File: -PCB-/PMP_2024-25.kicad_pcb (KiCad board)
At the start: 2 copper layers, 123 x 55.5 mm, 49 parts, among them J1 OUT, J2 5V, J3 GND, J4 CALIB, Q1 NPN 2N3904, Q2 NPN 2N3904, Q3 NPN MPSA42, Q4 NPN 2N3904

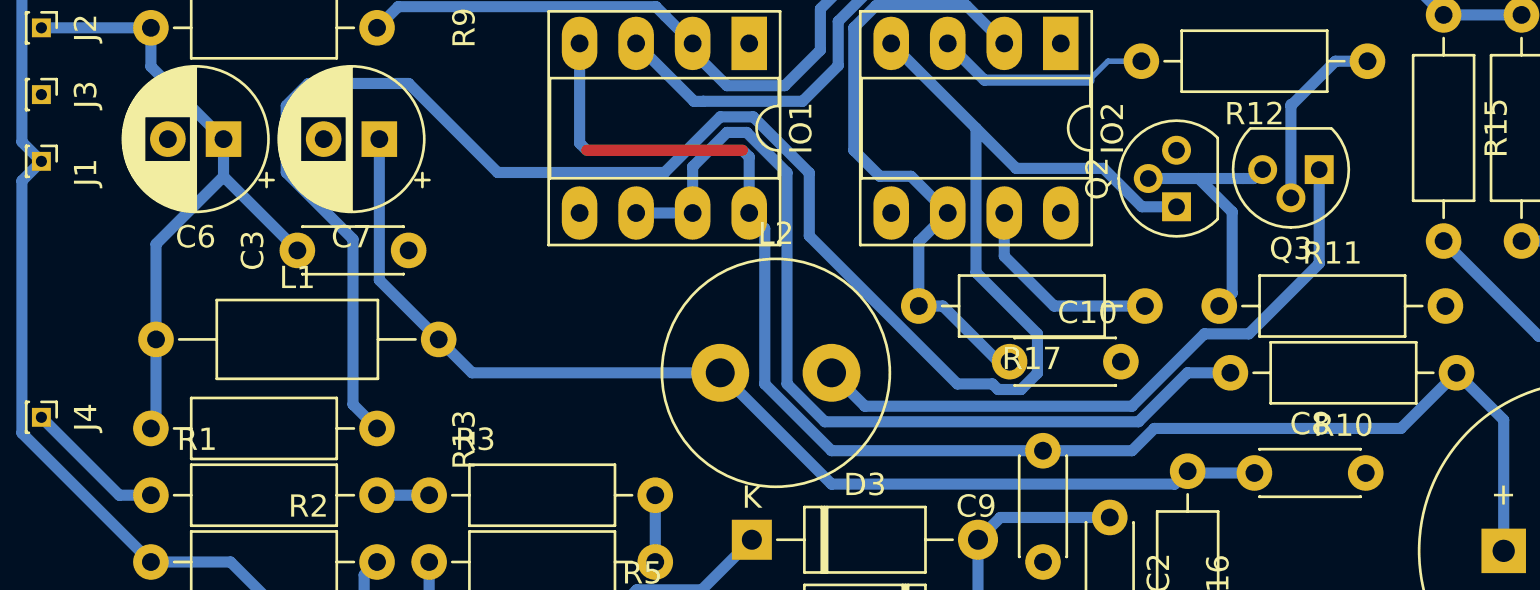
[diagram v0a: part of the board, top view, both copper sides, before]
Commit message: some edits
excel added too
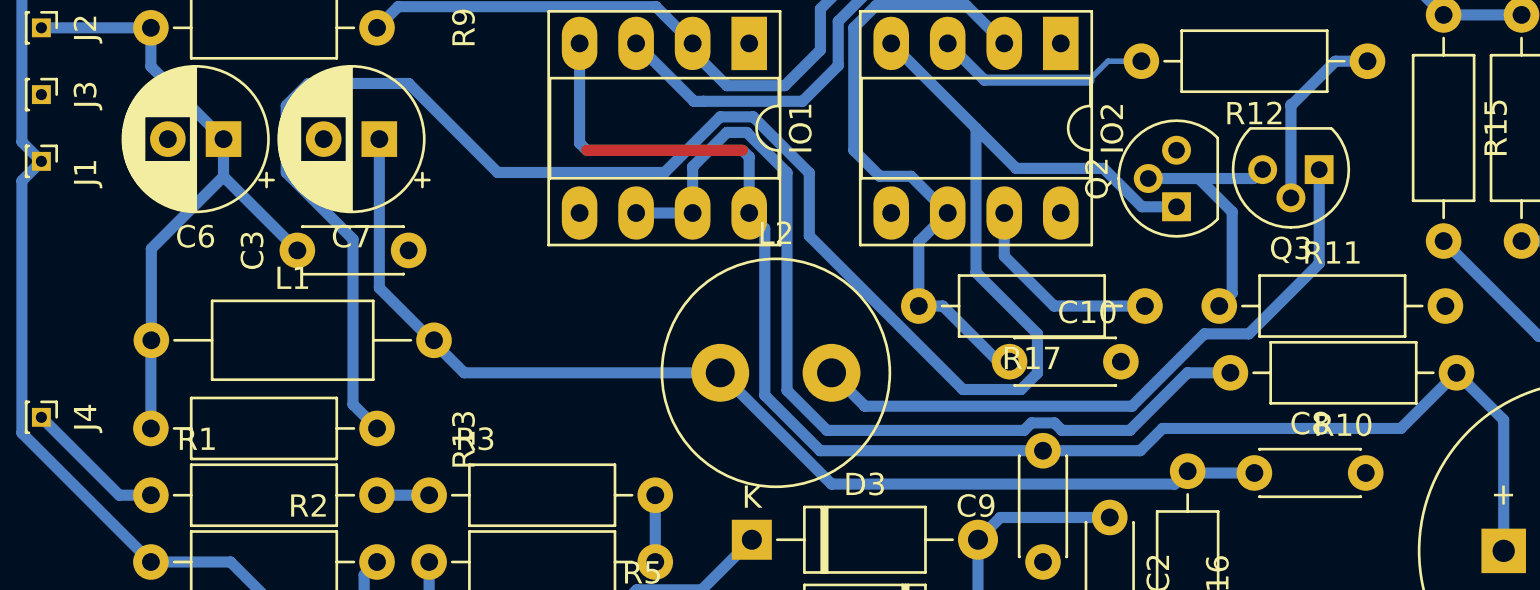
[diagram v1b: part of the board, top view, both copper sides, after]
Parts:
- moved L1 0.21 mm to (67.9, 65.0)
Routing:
- net Net-(IO1-DIS): track 41.3 -> 42.0 mm
- net VCC: track 30.3 -> 31.0 mm

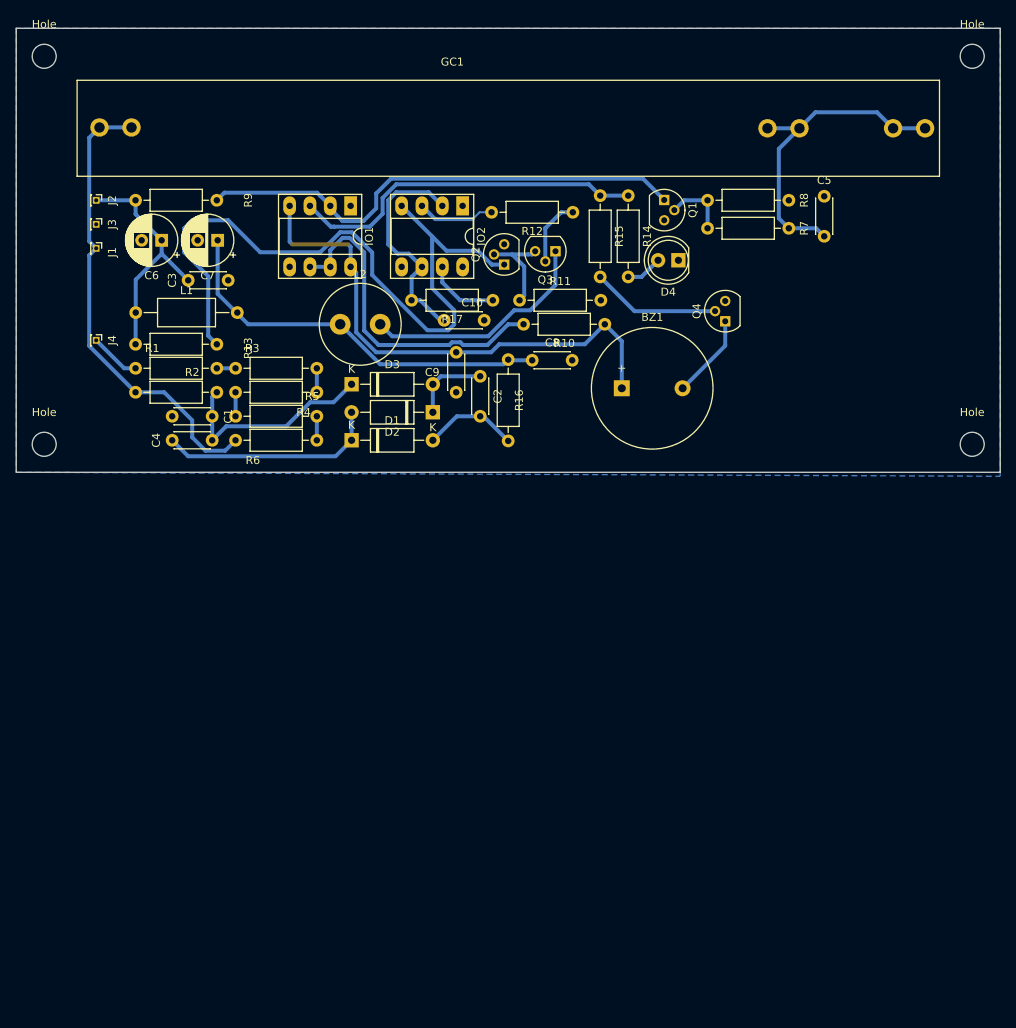
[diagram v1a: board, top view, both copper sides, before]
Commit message: PCB update
V2
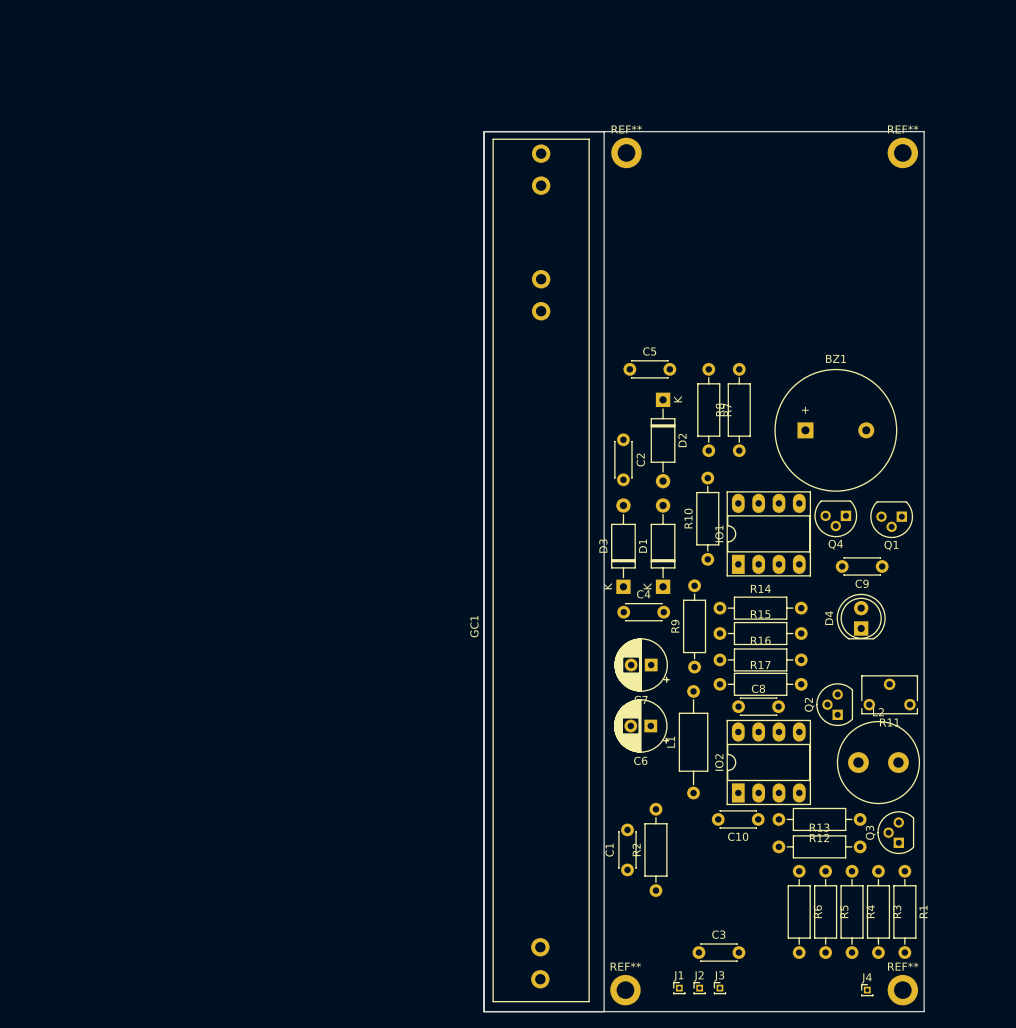
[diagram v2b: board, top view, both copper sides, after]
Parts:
- removed Hole (x4): MountingHole_3mm, MountingHole:MountingHole_3mm
- added REF**: MountingHole_2.2mm_M2_DIN965_Pad, MountingHole:MountingHole_2.2mm_M2_DIN965_Pad, F.Cu at (163.8, 149.7)
- added REF**: MountingHole_2.2mm_M2_DIN965_Pad, MountingHole:MountingHole_2.2mm_M2_DIN965_Pad, F.Cu at (129.2, 149.7)
- added REF**: MountingHole_2.2mm_M2_DIN965_Pad, MountingHole:MountingHole_2.2mm_M2_DIN965_Pad, F.Cu at (163.8, 45.1)
- added REF**: MountingHole_2.2mm_M2_DIN965_Pad, MountingHole:MountingHole_2.2mm_M2_DIN965_Pad, F.Cu at (129.3, 45.1)
- J4: value CALIB -> TEST
- R11: footprint Resistor_THT:R_Axial_DIN0207_L6.3mm_D2.5mm_P10.16mm_Horizontal -> Potentiometer_THT:Potentiometer_Bourns_3266W_Vertical
- R14: value ? -> 1k
- moved J4 126.1 mm to (159.4, 149.7), turned to 0 degrees
- moved J2 124.0 mm to (138.4, 149.5), turned to 0 degrees
- moved J3 123.3 mm to (141.0, 149.5), turned to 0 degrees
- moved GC1 123.2 mm to (119.6, 151.2), turned to 90 degrees
- moved J1 117.8 mm to (135.9, 149.5), turned to 0 degrees
- moved R1 106.5 mm to (164.1, 134.9), turned to -90 degrees
- moved C3 105.5 mm to (138.3, 145.0)
- moved R13 102.0 mm to (148.3, 131.8)
- moved R3 102.0 mm to (160.8, 134.9), turned to -90 degrees
- moved R4 97.6 mm to (157.5, 134.9), turned to -90 degrees
- moved R5 93.1 mm to (154.2, 134.9), turned to -90 degrees
- moved L1 92.0 mm to (137.7, 125.1), turned to 90 degrees
- moved R9 91.0 mm to (137.8, 109.3), turned to 90 degrees
- moved R2 90.1 mm to (133.0, 137.3), turned to 90 degrees
- moved R6 88.7 mm to (150.9, 134.9), turned to -90 degrees
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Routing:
- net RES: track 88.1 -> 0.00 mm
- net TRIG: track 62.4 -> 0.00 mm
- net Net-(BZ1-+): track 58.4 -> 0.00 mm
- net CALIB: track 58.1 -> 0.00 mm
- net Net-(IO2-VCC): track 50.1 -> 0.00 mm
- net Net-(IO1-Q): track 44.8 -> 0.00 mm
- net Net-(IO1-DIS): track 42.0 -> 0.00 mm
- net Net-(C5-Pad2): track 40.3 -> 0.00 mm
- net VCC: track 31.0 -> 0.06 mm
- net Net-(Q3-C): track 29.4 -> 0.00 mm
- net Net-(IO2-THR): track 29.0 -> 0.00 mm
- net Net-(D1-K): track 27.6 -> 0.00 mm
- net step_2: track 26.6 -> 0.00 mm
- net step_1: track 21.1 -> 0.00 mm
- net Net-(Q4-B): track 16.1 -> 0.00 mm
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- removed copper zone on B.Cu, net GND
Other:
- board size 123 x 55.5 mm -> 55 x 110 mm
